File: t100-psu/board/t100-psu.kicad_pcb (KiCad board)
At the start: 2 copper layers, 20 x 100 mm, 23 parts, among them J1 Conn_01x02_Female, J2 T100-IN, J3 T100-OUT, U1 FR8205, U2 FR8205

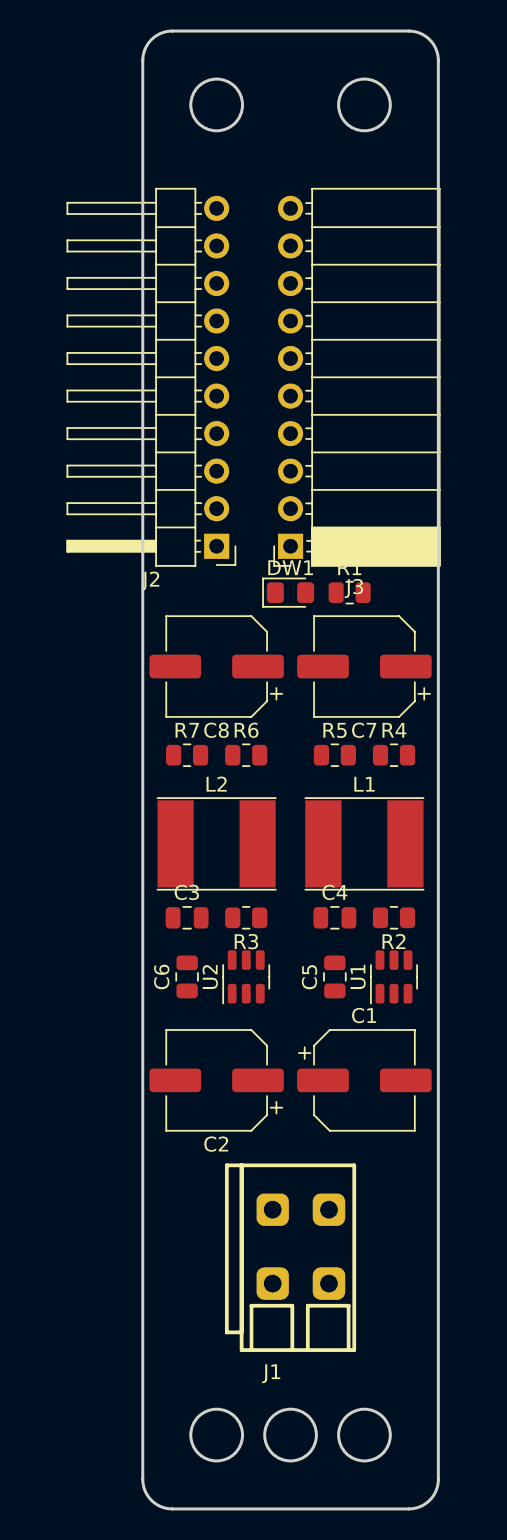
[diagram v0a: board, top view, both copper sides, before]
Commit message: WIP
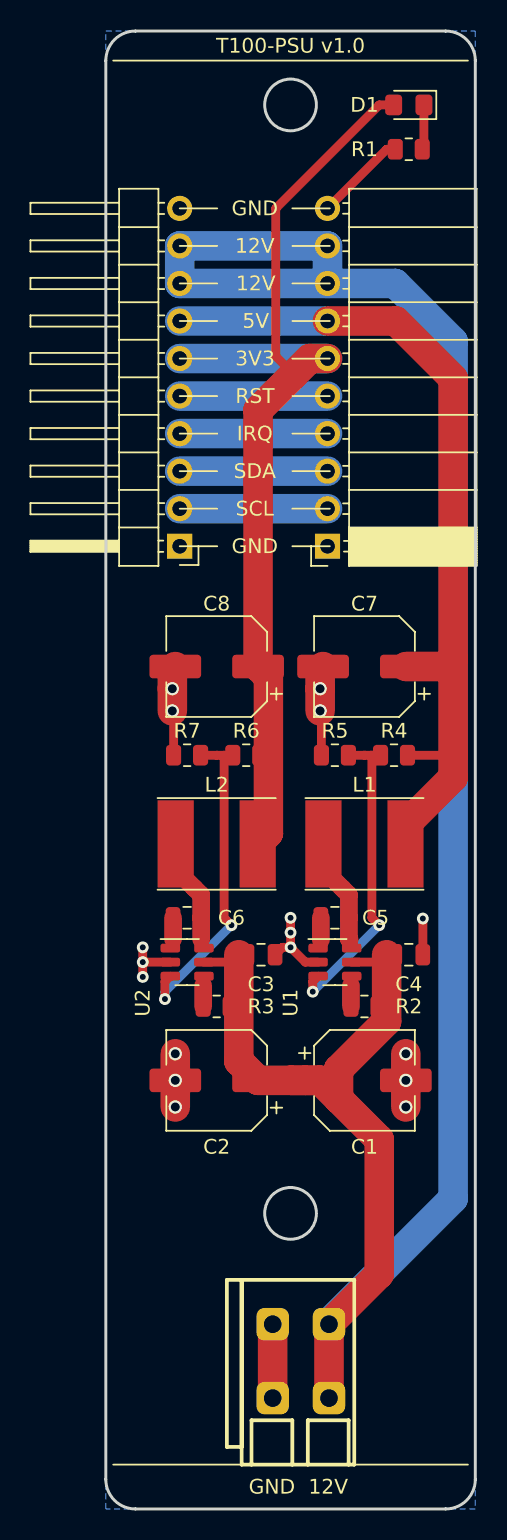
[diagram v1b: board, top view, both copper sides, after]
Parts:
- removed DW1: WHITE, LED_SMD:LED_0805_2012Metric_Pad1.15x1.40mm_HandSolder
- added D1: WHITE, LED_SMD:LED_0805_2012Metric_Pad1.15x1.40mm_HandSolder, F.Cu at (128.0, 60.0)
- moved R1 30.3 mm to (128.0, 63.0), turned to 180 degrees
- moved J1 7.75 mm to (118.8, 142.5)
- moved R2 6.32 mm to (125.0, 121.0), turned to 0 degrees
- moved R3 6.32 mm to (115.0, 121.0), turned to 0 degrees
- moved C3 5.59 mm to (118.0, 117.5), turned to 180 degrees
- moved C4 5.59 mm to (128.0, 117.5), turned to 180 degrees
- moved U1 4.12 mm to (123.0, 118.0), turned to 0 degrees
- moved U2 4.12 mm to (113.0, 118.0), turned to 0 degrees
- moved C5 4.00 mm to (123.0, 115.0), turned to 0 degrees
- moved C6 4.00 mm to (113.0, 115.0), turned to 0 degrees
- moved J2 2.50 mm to (112.5, 89.9)
- moved J3 2.50 mm to (122.5, 89.9)
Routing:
- net +12V: track 0.00 -> 160.8 mm
- net +3V3: track 0.00 -> 68.7 mm
- net +5V: track 0.00 -> 59.4 mm
- net GND: track 0.00 -> 43.5 mm, vias 0 -> 17
- net Net-(R6-Pad1): track 0.00 -> 22.4 mm, vias 0 -> 2
- net Net-(R4-Pad1): track 0.00 -> 21.4 mm, vias 0 -> 2
- net /SDA: track 0.00 -> 10.0 mm
- net /SCL: track 0.00 -> 10.0 mm
- net /RST: track 0.00 -> 10.0 mm
- net /IRQ: track 0.00 -> 10.0 mm
- net Net-(C5-Pad2): track 0.00 -> 7.24 mm
- net Net-(C6-Pad2): track 0.00 -> 7.16 mm
- net Net-(D1-Pad1): track 0.00 -> 3.05 mm
- net Net-(C5-Pad1): track 0.00 -> 1.50 mm
- net Net-(C6-Pad1): track 0.00 -> 1.45 mm
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- added copper zone on B.Cu, net GND
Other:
- board size 20 x 100 mm -> 25 x 100 mm
- board text added: "12V"
- board text added: "3V3"
- board text added: "5V"
- board text added: "GND"
- board text added: "IRQ"
- board text added: "RST"
- board text added: "SCL"
- board text added: "SDA"
- board text added: "T100-PSU v1.0"
